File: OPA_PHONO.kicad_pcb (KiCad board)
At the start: 4 copper layers, 99 x 30 mm, 59 parts, among them J2 Conn_Coaxial_x2, J3 Conn_Coaxial_x2, J4 USB_C_Receptacle_USB2.0, U1 OPA1644AxD, U2 OPA1612AxD, U3 LTC3265xDHC

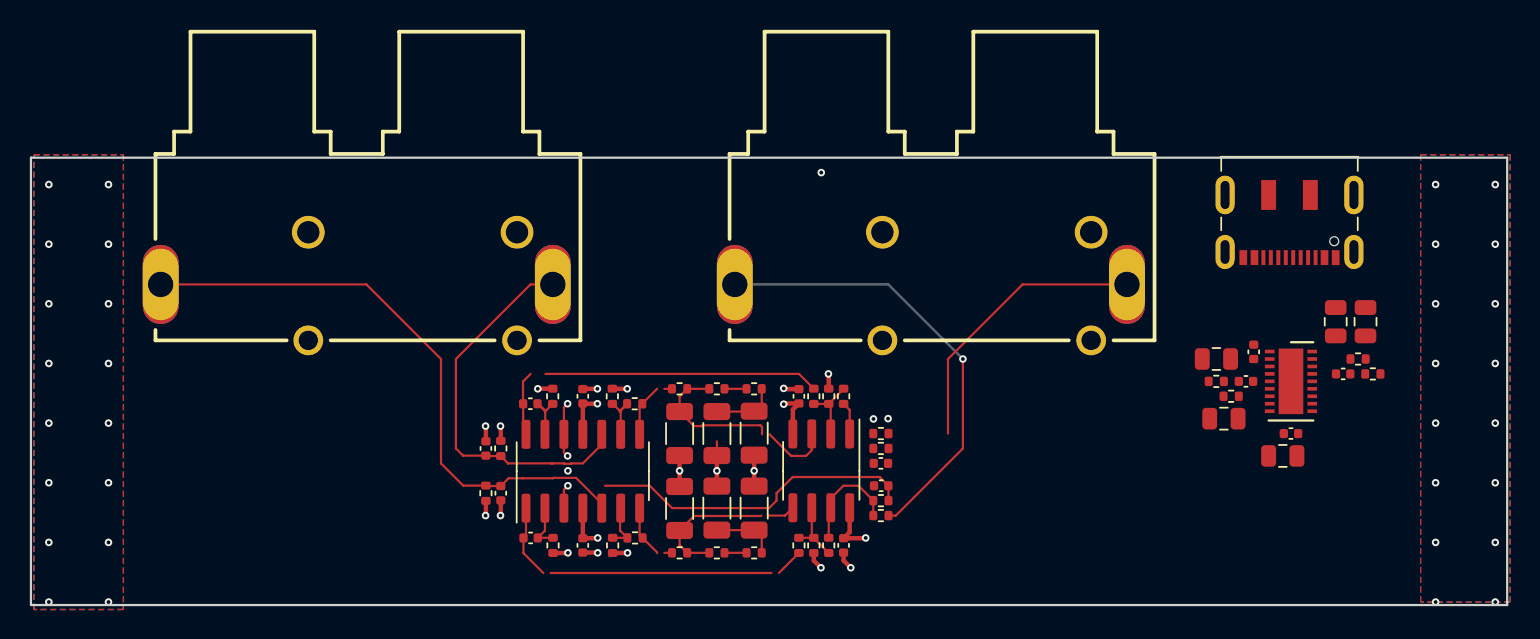
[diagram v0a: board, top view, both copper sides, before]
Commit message: update layout
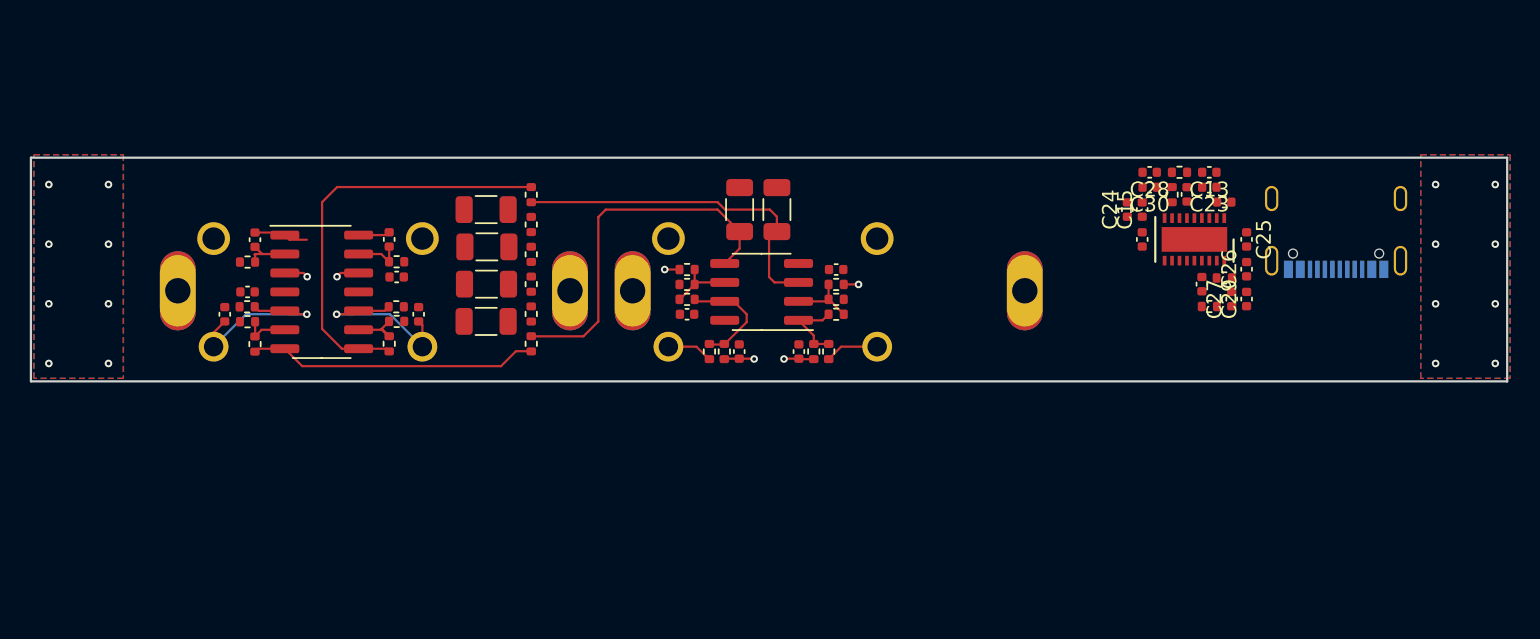
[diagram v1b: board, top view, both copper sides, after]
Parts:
- removed J3: Conn_Coaxial_x2, OPA_PHONO:PJRAS2X1S01X
- added C26: 4.7u, Capacitor_SMD:C_0402_1005Metric, F.Cu at (196.3, 83.7)
- added C27: 4.7u, Capacitor_SMD:C_0402_1005Metric, F.Cu at (195.3, 85.7)
- added C28: 4.7u, Capacitor_SMD:C_0402_1005Metric, F.Cu at (189.8, 77.2)
- added C29: 4.7u, Capacitor_SMD:C_0402_1005Metric, F.Cu at (196.3, 85.7)
- added C30: 4.7u, Capacitor_SMD:C_0402_1005Metric, F.Cu at (189.8, 78.2)
- added Je: Conn_Coaxial_x2, OPA_PHONO:PJRAS2X1S01X, B.Cu at (168.3, 85.2)
- C13, C15, C23, C24, C25: value 10u -> 4.7u; footprint Capacitor_SMD:C_0805_2012Metric -> Capacitor_SMD:C_0402_1005Metric
- J2: moved to B.Cu
- J4: value USB_C_Receptacle_USB2.0 -> UJC-HP-3-SMT-TR; footprint Connector_USB:USB_C_Receptacle_JAE_DX07S016JA1R1500 -> Connector_USB:USB_C_Receptacle_Palconn_UTC16-G; moved to B.Cu
- moved R15 28.7 mm to (129.3, 87.2), turned to 0 degrees
- moved R14 28.6 mm to (129.8, 88.7), turned to 90 degrees
- moved C19 28.2 mm to (129.3, 85.2), turned to 0 degrees
- moved R22 27.9 mm to (129.3, 83.2), turned to 0 degrees
- moved C11 27.2 mm to (129.8, 81.7), turned to -90 degrees
- moved R18 23.4 mm to (148.3, 84.7), turned to 90 degrees
- moved C7 22.1 mm to (127.8, 86.7), turned to 90 degrees
- moved C9 21.9 mm to (145.3, 87.2), turned to 180 degrees
- moved C3 21.9 mm to (145.4, 82.2), turned to 180 degrees
- moved C2 21.6 mm to (145.3, 79.7), turned to 180 degrees
- moved C8 21.5 mm to (145.3, 84.7), turned to 180 degrees
- moved U1 21.2 mm to (134.3, 85.2), turned to 0 degrees
- moved C10 20.4 mm to (162.3, 79.7)
- moved R13 20.3 mm to (129.3, 86.2), turned to 0 degrees
- moved R17 20.3 mm to (148.3, 86.7), turned to -90 degrees
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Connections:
- net /LEFT/FB3 renamed /LEFT/FBTRIM
- net /LEFT/OUT3 renamed /LEFT/TRIM
- net /RIGHT/FB3 renamed /RIGHT/FBTRIM
- net /RIGHT/OUT3 renamed /RIGHT/TRIM
- C23 pad 2: /POWER/VOUTP -> /POWER/VIN
- C24 pad 2: +12V -> /POWER/VOUTN
- C25 pad 1: -12V -> GND
- C25 pad 2: GND -> /POWER/VOUTP
- J2 pad 1: /IN_R -> (no net)
- J2 pad 2: /IN_L -> (no net)
- J2 pad S1: (no net) -> GND
- J2 pad S2: (no net) -> GND
- J2 pad T1: (no net) -> /IN_L
- J2 pad T2: (no net) -> /IN_R
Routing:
- net /IN_L: track 40.5 -> 12.9 mm, vias 0 -> 1
- net /OUT_L: track 30.2 -> 3.11 mm, vias 1 -> 0
- net /RIGHT/OUT1: track 4.26 -> 28.1 mm
- net GND: track 21.9 -> 0.00 mm, vias 52 -> 16
- net /LEFT/OUT_RC: track 23.6 -> 3.62 mm, vias 1 -> 2
- net /RIGHT/TRIM: track 23.0 -> 3.12 mm, vias 0 -> 1
- net /LEFT/TRIM: track 21.7 -> 4.66 mm, vias 0 -> 1
- net /OUT_R: track 19.1 -> 3.60 mm
- net /LEFT/OUT1: track 3.99 -> 19.2 mm
- net /LEFT/RIAA: track 10.9 -> 24.8 mm
- net /IN_R: track 25.3 -> 12.1 mm, vias 0 -> 1
- net /RIGHT/RIAA: track 14.4 -> 23.3 mm
- net +12V: track 6.73 -> 0.00 mm, vias 2 -> 0
- net -12V: track 6.31 -> 0.00 mm, vias 2 -> 0
- net /LEFT/RIAA_RC: track 4.24 -> 0.00 mm
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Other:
- board size 99 x 30 mm -> 99 x 15 mm
